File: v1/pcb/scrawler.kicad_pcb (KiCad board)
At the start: 2 copper layers, 161.7 x 126 mm, 99 parts, among them J2 MJ-4PP-9, J3 OLED, SW10A1 SW_PUSH, SW10B1 SW_PUSH, SW11A1 SW_PUSH, SW11B1 SW_PUSH, SW12A1 SW_PUSH, SW12B1 SW_PUSH, SW13A1 SW_PUSH, SW13B1 SW_PUSH, SW14A1 SW_PUSH, SW14B1 SW_PUSH, SW15A1 SW_PUSH, SW15B1 SW_PUSH, SW16A1 SW_PUSH, SW16B1 SW_PUSH, SW17A1 SW_PUSH, SW17B1 SW_PUSH, SW18A1 SW_PUSH, SW18B1 SW_PUSH, SW19A1 SW_PUSH, SW19B1 SW_PUSH, SW1A1 SW_PUSH, SW1B1 SW_PUSH, SW20A1 SW_PUSH, SW20B1 SW_PUSH, SW21A1 SW_PUSH, SW21B1 SW_PUSH, SW22A1 SW_PUSH, SW22B1 SW_PUSH, SW24A1 SW_PUSH, SW24B1 SW_PUSH, SW25A1 SW_PUSH, SW25B1 SW_PUSH, SW26 Rotary_Encoder_Switch, SW26A1 SW_PUSH, SW26B1 SW_PUSH, SW2A1 SW_PUSH, SW2B1 SW_PUSH, SW3A1 SW_PUSH, SW3B1 SW_PUSH, SW4A1 SW_PUSH, SW4B1 SW_PUSH, SW5A1 SW_PUSH, SW5B1 SW_PUSH, SW6A1 SW_PUSH, SW6B1 SW_PUSH, SW7A1 SW_PUSH, SW7B1 SW_PUSH, SW8A1 SW_PUSH, SW8B1 SW_PUSH, SW9A1 SW_PUSH, SW9B1 SW_PUSH, U1 ProMicro

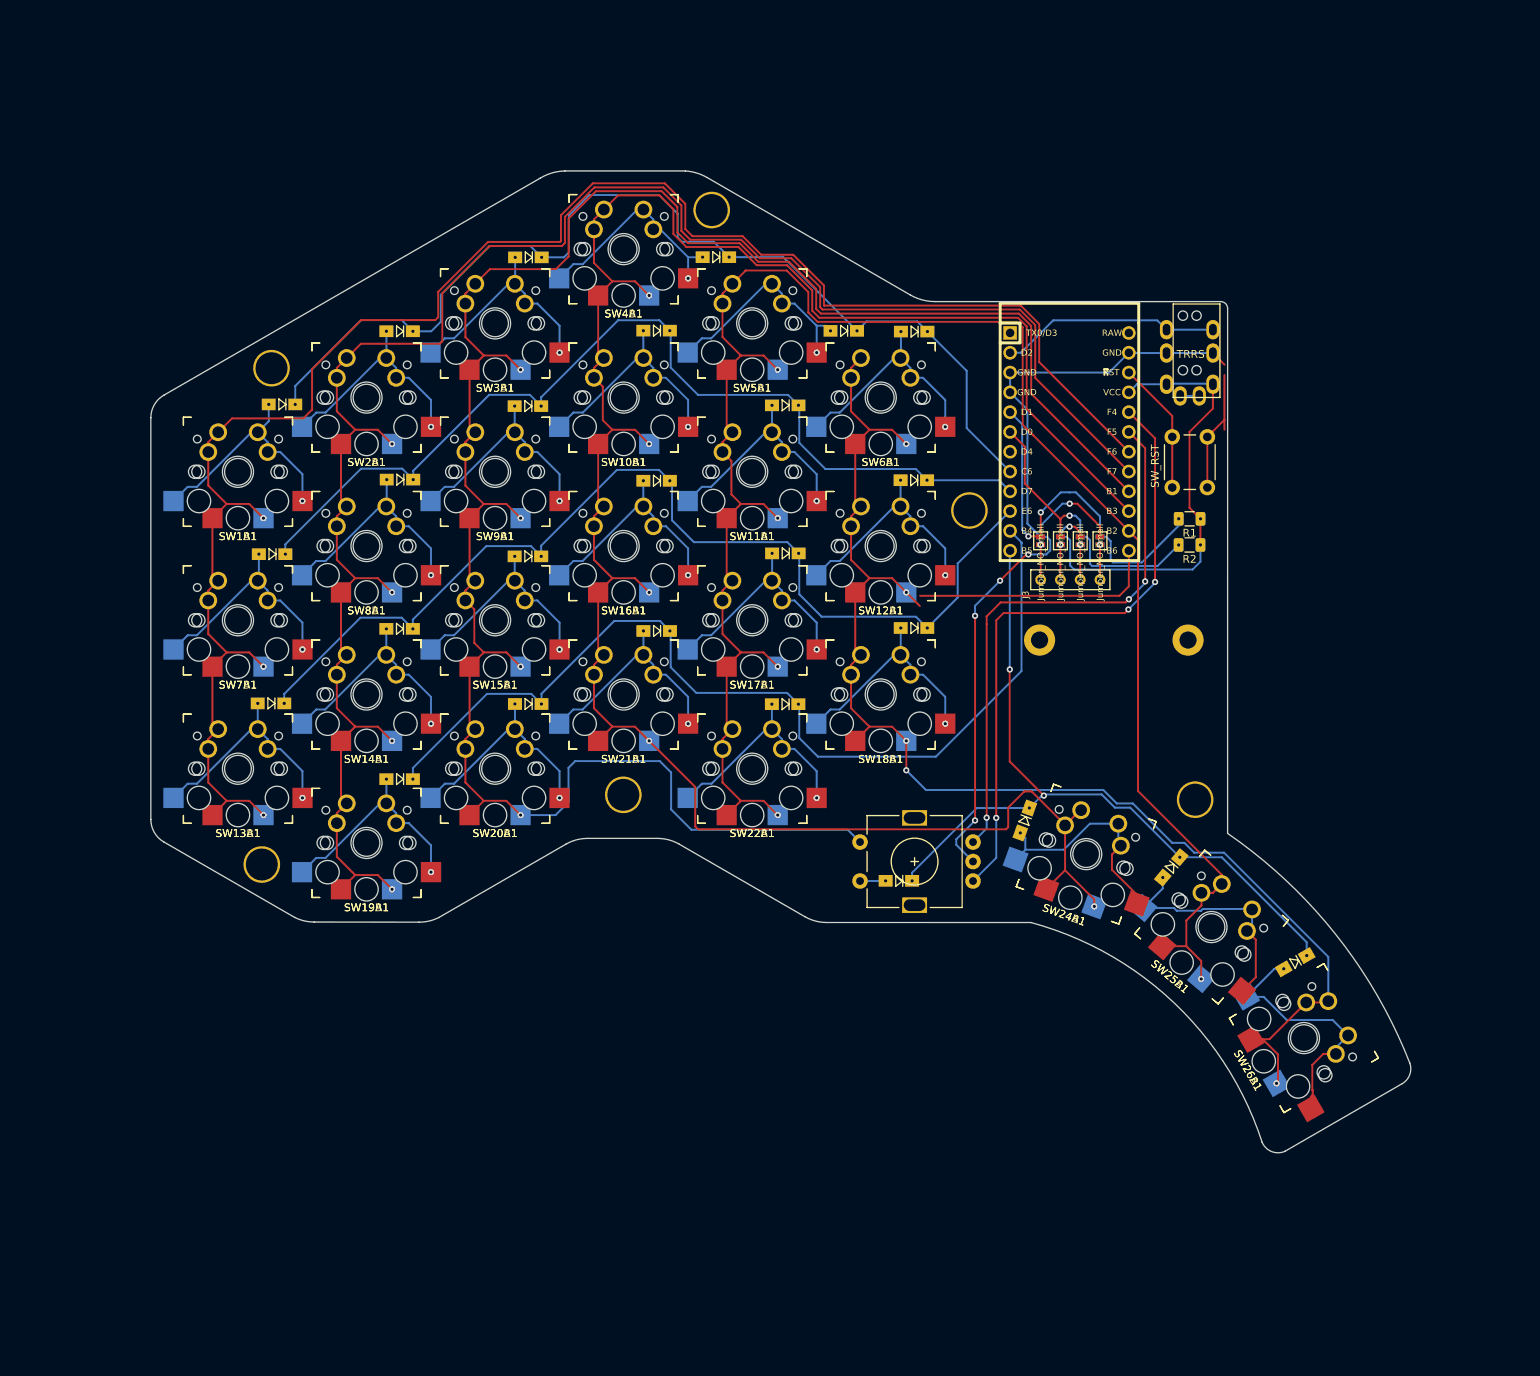
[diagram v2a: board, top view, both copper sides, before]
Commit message: generated gerber files
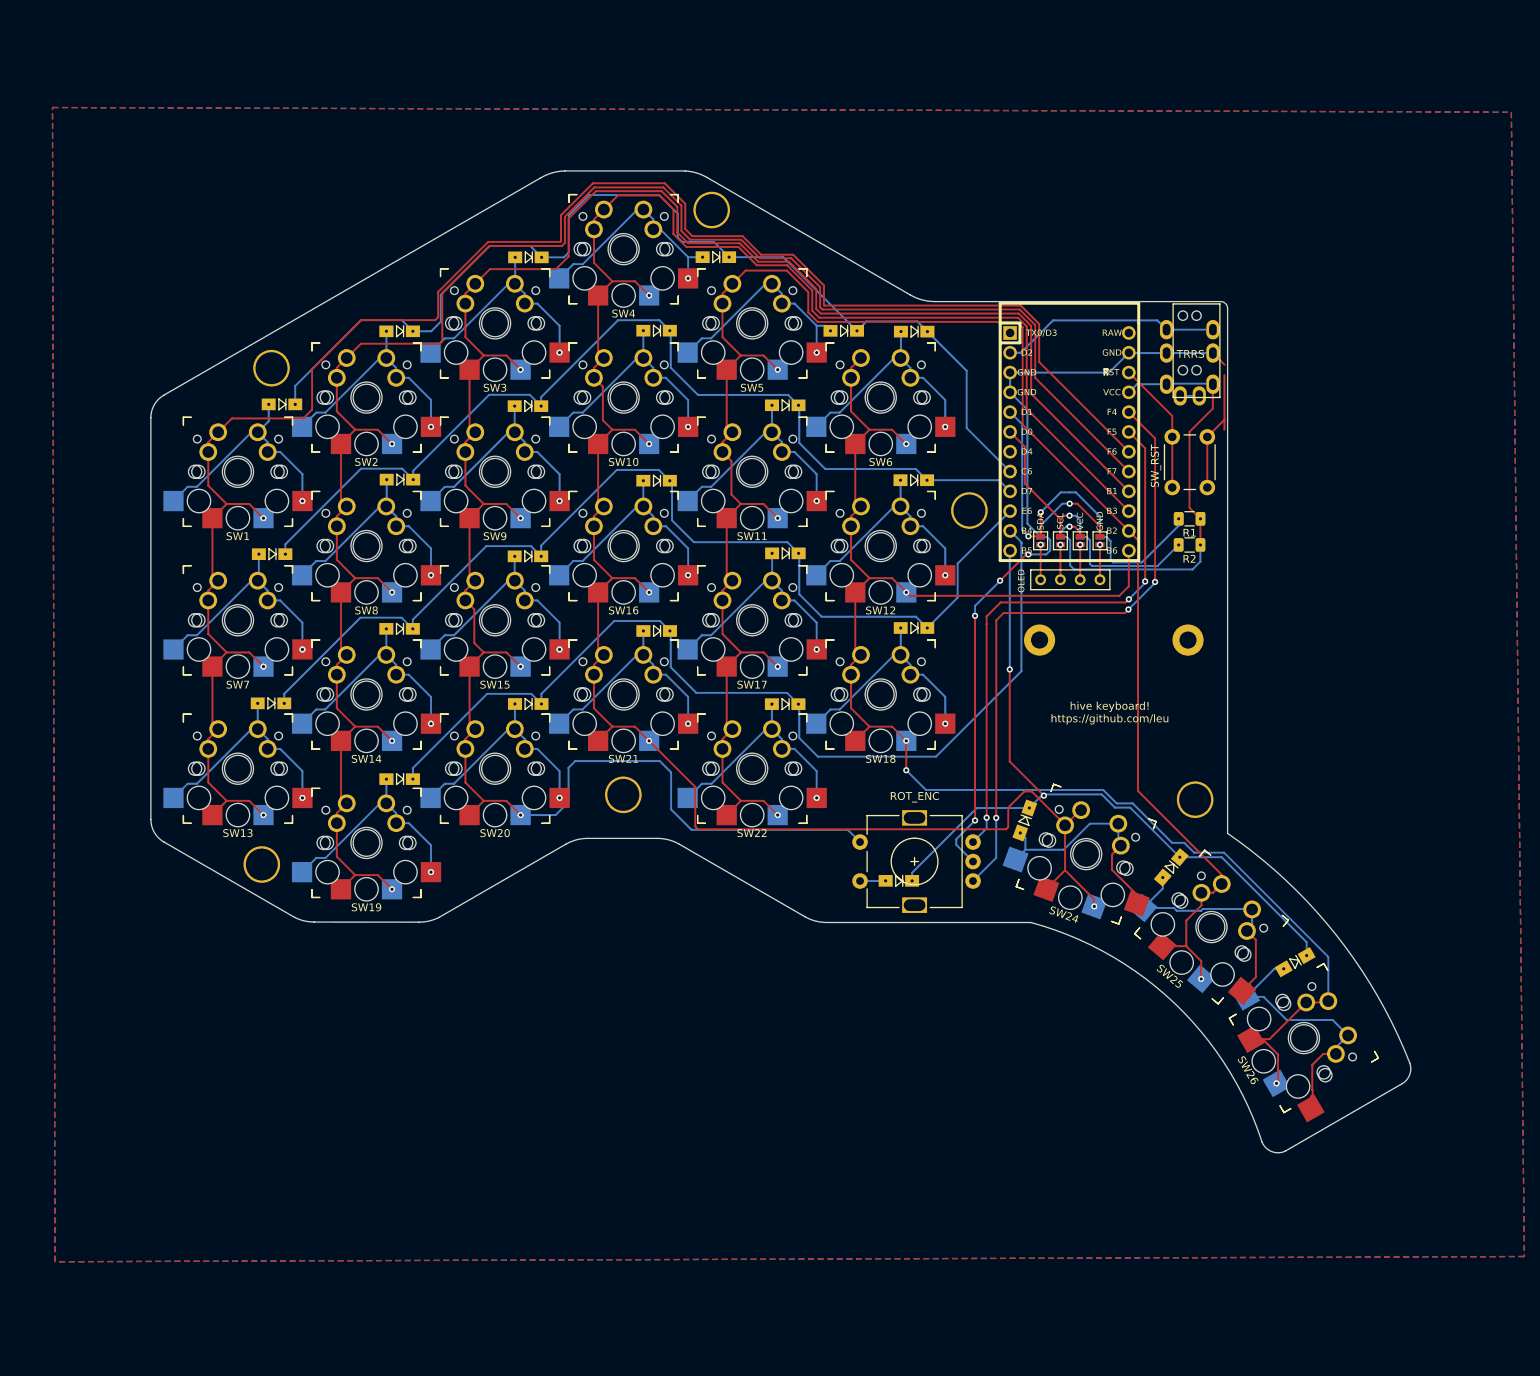
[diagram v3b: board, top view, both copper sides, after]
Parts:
- JP1, JP8: value Jumper_NO_Small -> GND
- JP2, JP7: value Jumper_NO_Small -> VCC
- JP3, JP6: value Jumper_NO_Small -> SCL
- JP4, JP5: value Jumper_NO_Small -> SDA
- renumbered J3 to OLED, SW26 to ROT_ENC, SW1A1 to SW1, SW10A1 to SW10, SW11A1 to SW11, SW12A1 to SW12, SW13A1 to SW13, SW14A1 to SW14, SW15A1 to SW15, SW16A1 to SW16, SW17A1 to SW17, SW18A1 to SW18, SW19A1 to SW19, SW2A1 to SW2, SW20A1 to SW20, SW21A1 to SW21, SW22A1 to SW22, SW24A1 to SW24, SW25A1 to SW25, SW26A1 to SW26, SW3A1 to SW3, SW4A1 to SW4, SW5A1 to SW5, SW6A1 to SW6, SW7A1 to SW7, SW8A1 to SW8, SW9A1 to SW9
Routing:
- net COL5: track 199.3 -> 198.8 mm
- added copper zone on B.Cu, net GND
- added copper zone on F.Cu, net GND
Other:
- board text added: "hive keyboard! https://github.com/leu"
